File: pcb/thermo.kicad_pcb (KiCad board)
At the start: 2 copper layers, 26 parts, among them J1 DB15_Female, J2 Barrel_Jack, U1 BME280

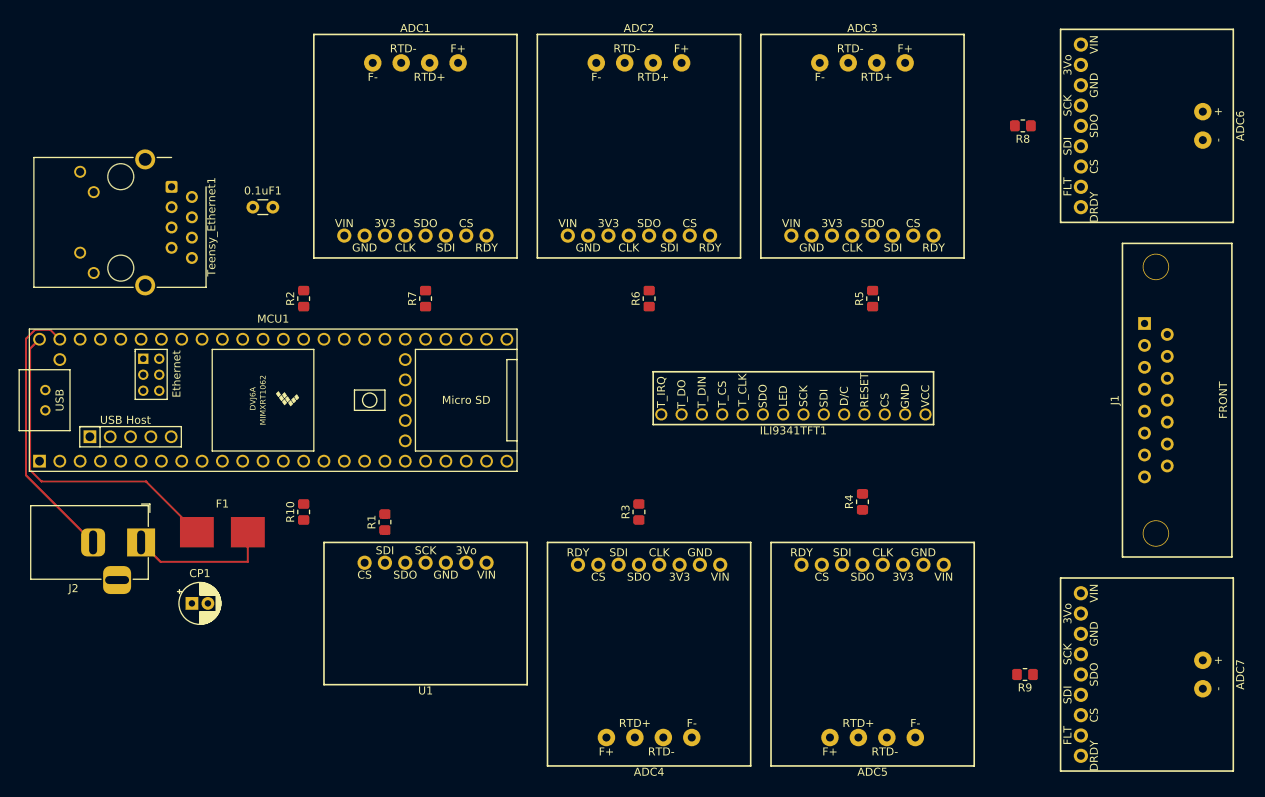
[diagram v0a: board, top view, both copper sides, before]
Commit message: Latest upload for Brian to check
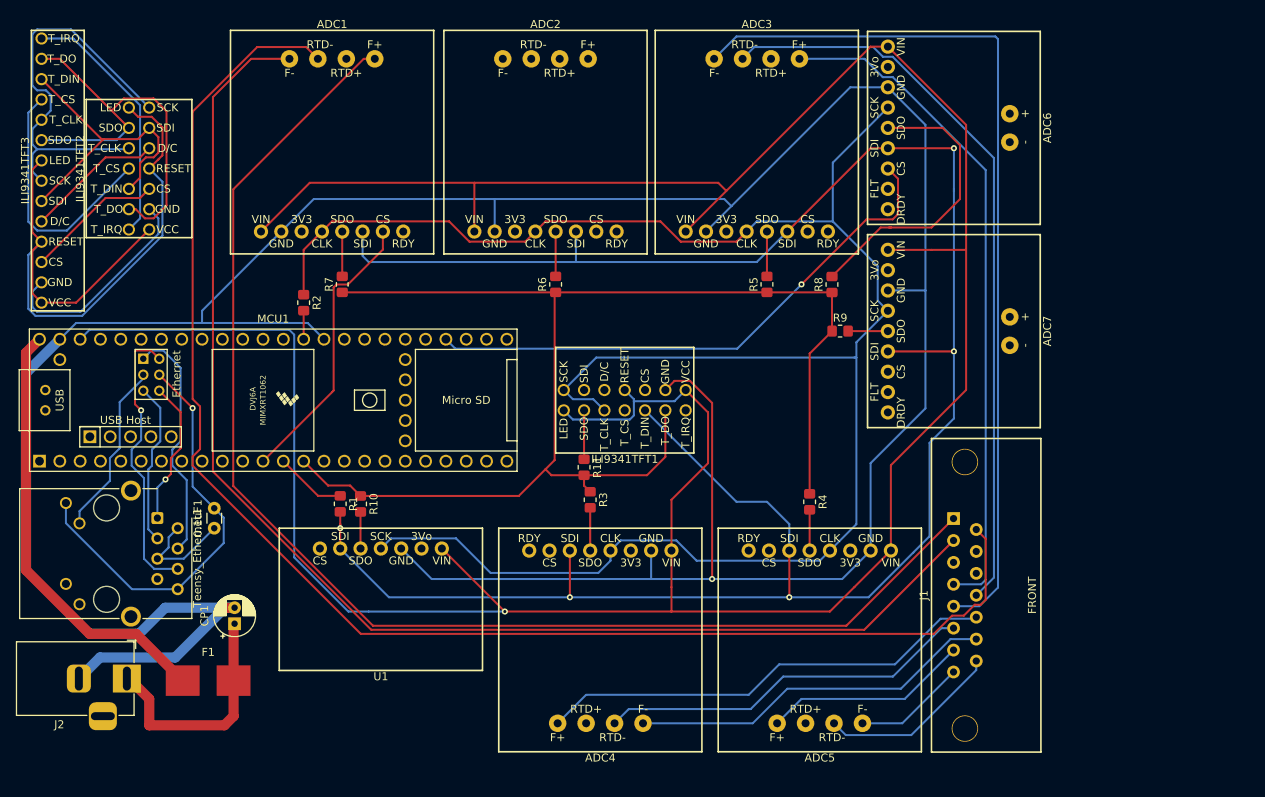
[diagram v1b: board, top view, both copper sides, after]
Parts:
- added ILI9341TFT2: Conn_01x14, Thermometry:ILI9341_2x7_connector, F.Cu at (32.8, 79.0)
- added ILI9341TFT3: Conn_01x14, Thermometry:ILI9341_1x14_connector, F.Cu at (20.6, 79.2)
- added R11: 22, Resistor_SMD:R_0805_2012Metric_Pad1.20x1.40mm_HandSolder, F.Cu at (88.4, 116.3)
- ILI9341TFT1: footprint Thermometry:ILI9341_1x14_connector -> Thermometry:ILI9341_2x7_connector
- moved ADC7 49.2 mm to (134.6, 99.3)
- moved R9 48.8 mm to (120.4, 99.3), turned to 0 degrees
- moved Teensy_Ethernet1 41.4 mm to (35.1, 122.7)
- moved 0.1uF1 40.4 mm to (42.2, 124.0), turned to 90 degrees
- moved J1 34.1 mm to (137.4, 132.3)
- moved R8 31.0 mm to (119.4, 93.5), turned to 90 degrees
- moved ADC6 24.1 mm to (134.6, 73.9)
- moved ILI9341TFT1 21.2 mm to (93.5, 108.0)
- moved F1 18.6 mm to (41.4, 143.0)
- moved J2 17.1 mm to (31.2, 142.7)
- moved R5 13.3 mm to (111.3, 93.5)
- moved ADC3 13.2 mm to (110.0, 75.7)
- moved R6 11.8 mm to (84.8, 93.5)
- moved ADC2 11.7 mm to (83.6, 75.7)
- moved R7 10.6 mm to (58.2, 93.5)
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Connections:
- ILI9341TFT1 pad 9: /SDO -> Net-(ILI9341TFT1-Pad9)
- MCU1 pad 30: Net-(MCU1-Pad30) -> /CS_8
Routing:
- net +3V3: track 0.00 -> 468.3 mm, vias 0 -> 1
- net GND: track 34.1 -> 417.7 mm, vias 0 -> 1
- net /SDI: track 0.00 -> 306.6 mm, vias 0 -> 5
- net /CLK: track 0.00 -> 300.6 mm
- net /SDO: track 0.00 -> 220.3 mm
- net Net-(ADC1-Pad10): track 0.00 -> 183.5 mm
- net Net-(ADC1-Pad12): track 0.00 -> 164.4 mm
- net Net-(ADC1-Pad9): track 0.00 -> 163.7 mm
- net Net-(ADC3-Pad9): track 0.00 -> 111.9 mm
- net Net-(ADC3-Pad10): track 0.00 -> 93.4 mm
- net Net-(ADC3-Pad12): track 0.00 -> 84.5 mm
- net /CS_6: track 0.00 -> 70.2 mm, vias 0 -> 1
- net Net-(ADC4-Pad12): track 0.00 -> 57.8 mm
- net Net-(0.1uF1-Pad2): track 0.00 -> 52.4 mm, vias 0 -> 1
- net Net-(ADC4-Pad10): track 0.00 -> 47.3 mm
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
